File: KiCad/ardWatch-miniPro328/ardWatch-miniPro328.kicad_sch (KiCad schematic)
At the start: 8 parts, among them J1 2-pin_power_input_header, U1 Arduino_Mini_Pro, U2 KY-040_Rotary_Encoder, U3 ST7735_1.8"_TFT_128x160, U4 DS3231_RTC_module

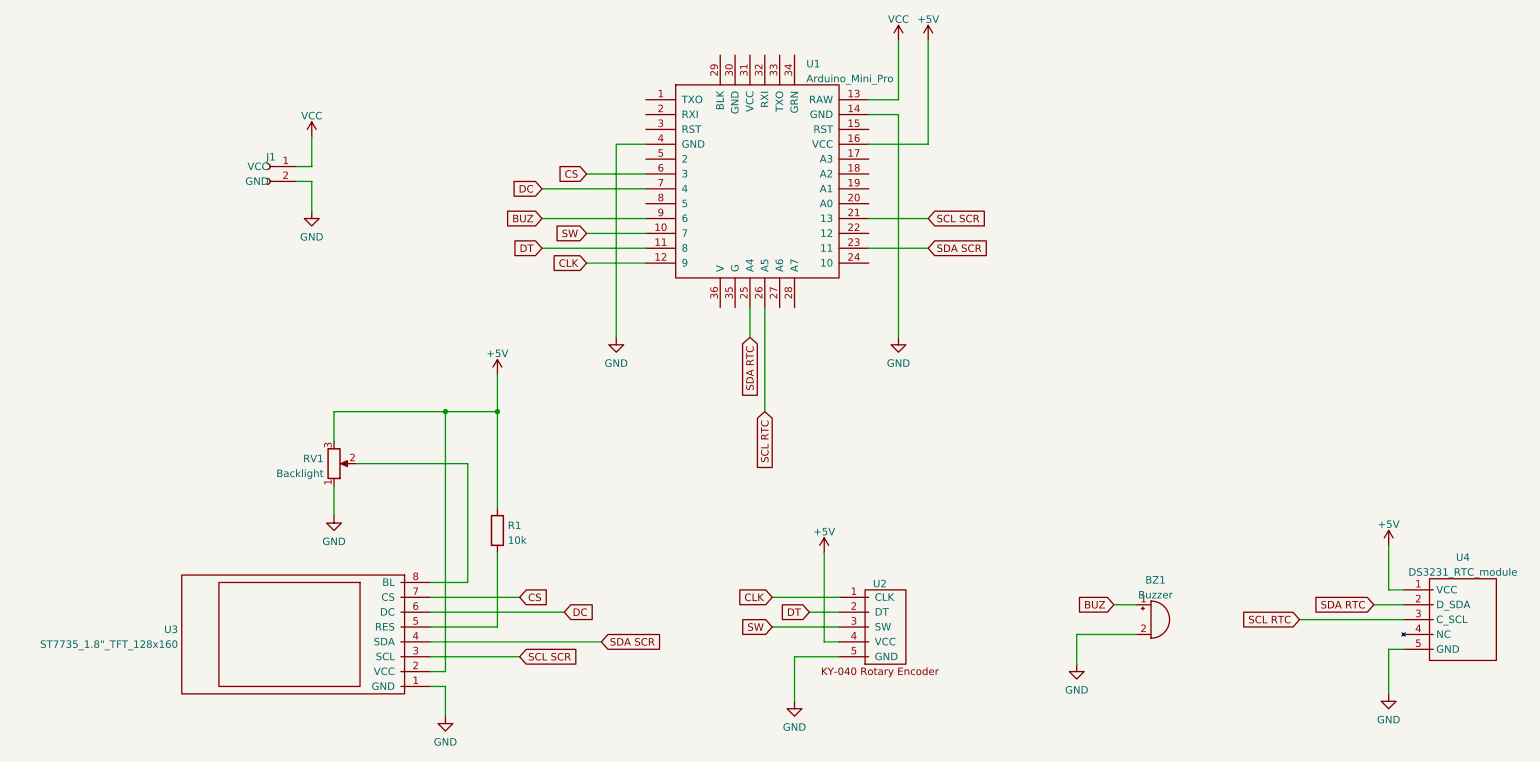
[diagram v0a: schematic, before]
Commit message: kicad v8
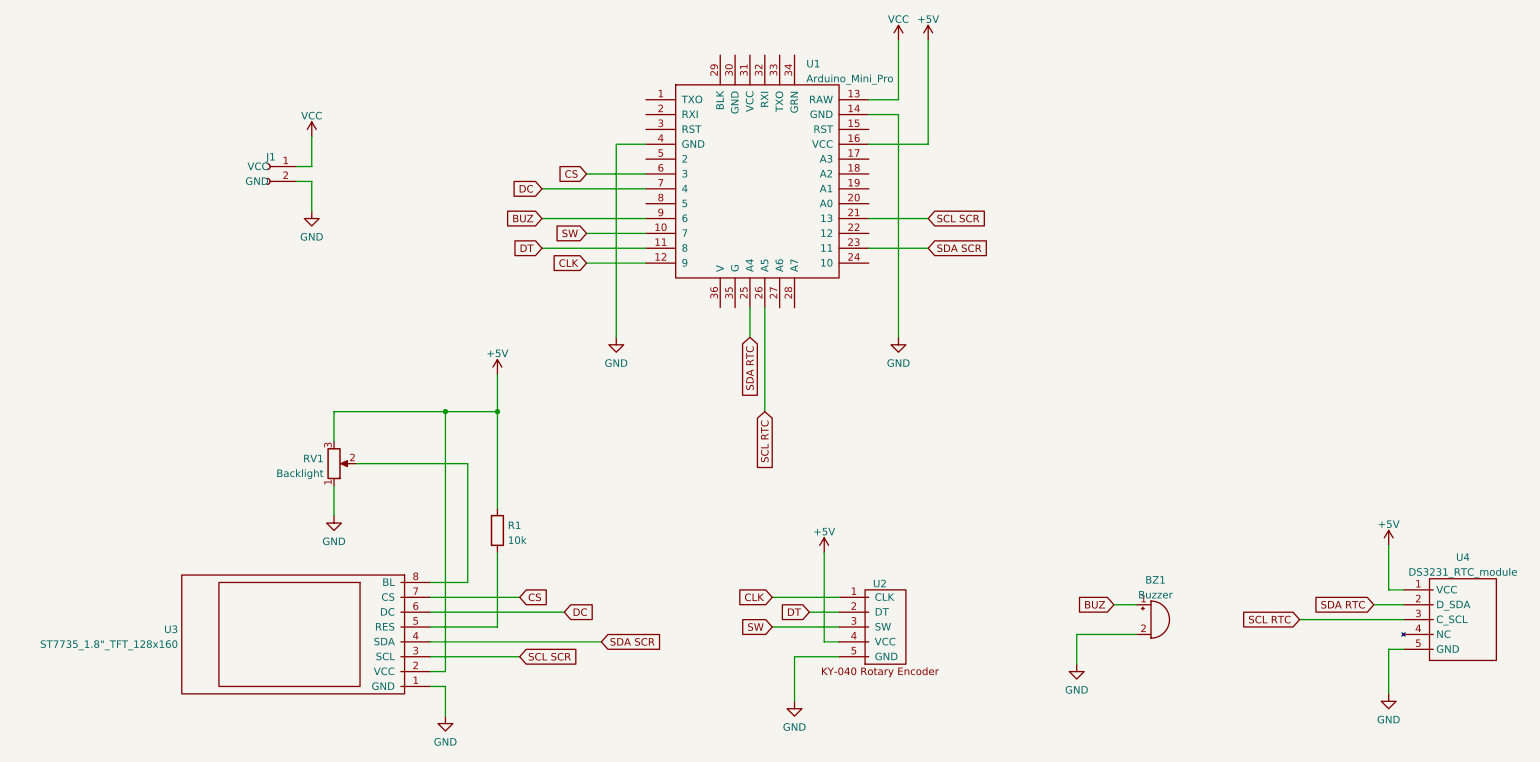
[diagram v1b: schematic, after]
